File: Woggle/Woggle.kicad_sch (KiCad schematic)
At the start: 23 parts, among them SW1 SW_SPDT, SW2 Sequance, U1 ATtiny85-20P

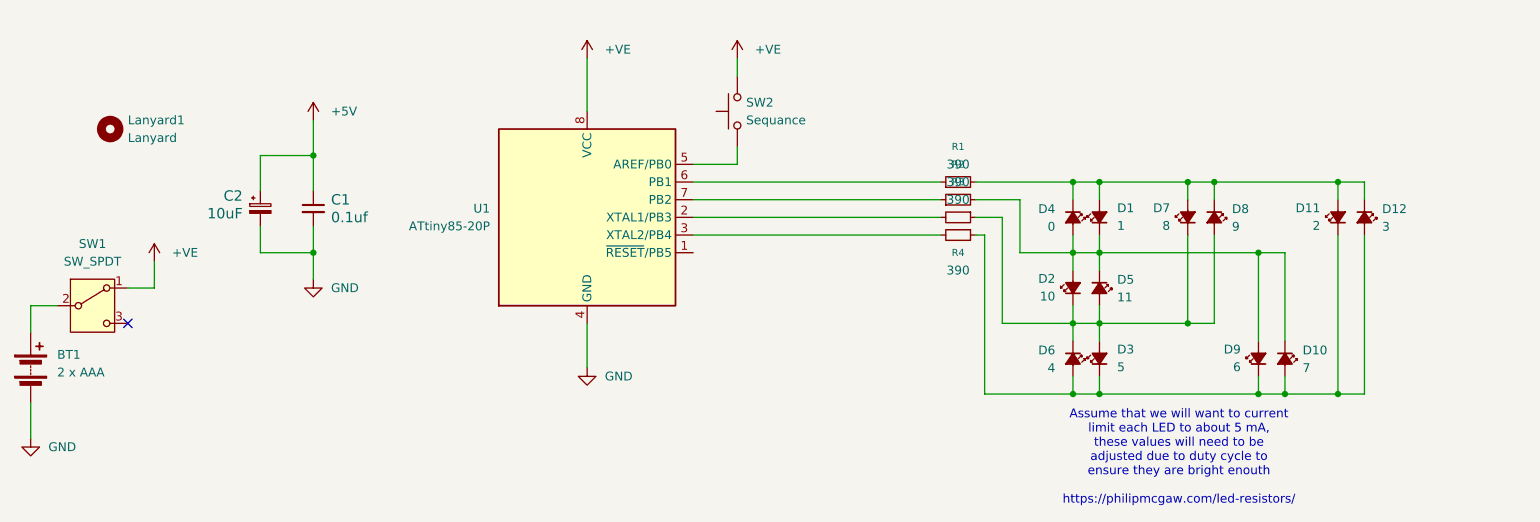
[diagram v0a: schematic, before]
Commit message: .
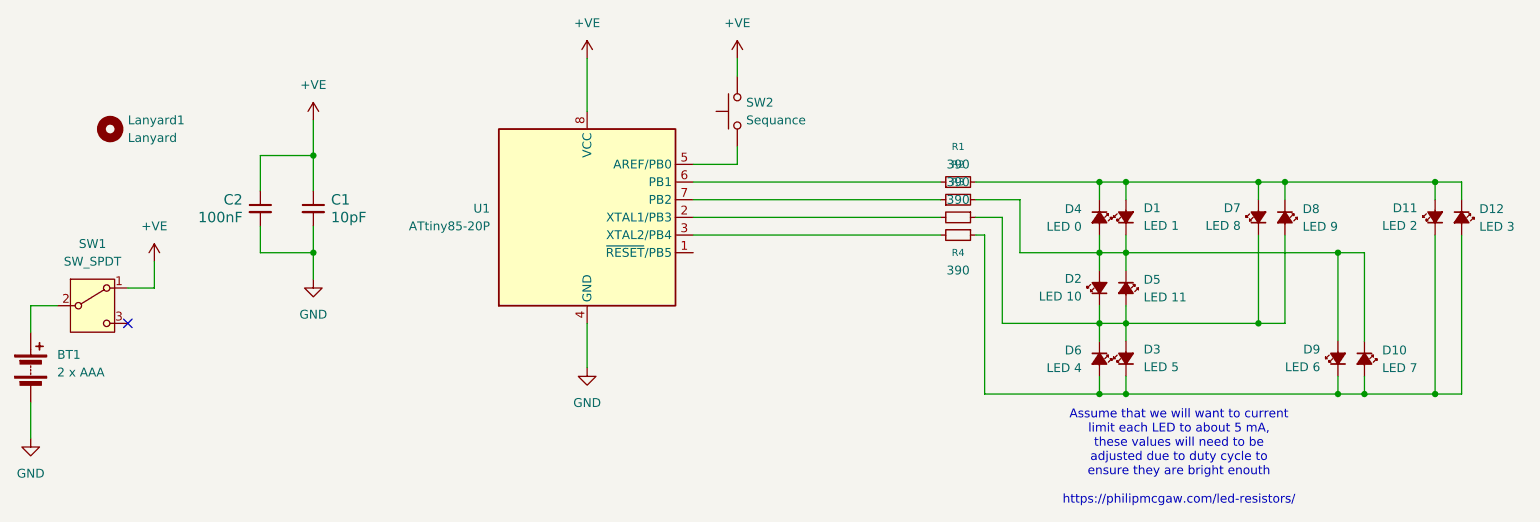
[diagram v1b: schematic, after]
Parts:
- removed C2: 10uF, Capacitors_THT:CP_Radial_D5.0mm_P2.50mm, symbol Device:C_Polarized_Small
- added C2: 100nF, Capacitor_THT:C_Disc_D4.7mm_W2.5mm_P5.00mm, symbol Device:C_Small
- C1: value 0.1uf -> 10pF; footprint Franzininho:C025-025X050 -> Capacitor_THT:C_Disc_D4.7mm_W2.5mm_P5.00mm; code (none) -> 100
- D1: value 1 -> LED 1
- D10: value 7 -> LED 7
- D11: value 2 -> LED 2
- D12: value 3 -> LED 3
- D2: value 10 -> LED 10
- D3: value 5 -> LED 5
- D4: value 0 -> LED 0
- D5: value 11 -> LED 11
- D6: value 4 -> LED 4
- D7: value 8 -> LED 8
- D8: value 9 -> LED 9
- D9: value 6 -> LED 6
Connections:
- net +5V is gone; now on net +VE: C1.1
- net +VE: now also C2.1
- net GND: now also C2.2
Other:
- moved on the sheet: D1, D10, D11, D12, D2, D3, D4, D5, D6, D7, D8, D9

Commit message: .
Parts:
- BT1: footprint Scouts:2 x AAA battery cell holder -> Scouts:Scouts - 2 x AAA battery cell holder
- D1, D10, D11, D12, D2, D3, D4, D5, D6, D7, D8, D9: footprint Scouts:5mm LED -> Scouts:Scouts - 5mm LED
- R1, R2, R3, R4: footprint Resistor_THT:R_Axial_DIN0207_L6.3mm_D2.5mm_P10.16mm_Horizontal -> Scouts:Scouts - Resistor (10.16mm)
- U1: footprint Scouts:DIP 8 -> Scouts:Scouts - DIP 8
